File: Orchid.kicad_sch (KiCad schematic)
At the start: 122 parts, among them U1 nice_nano, U2 nice_nano

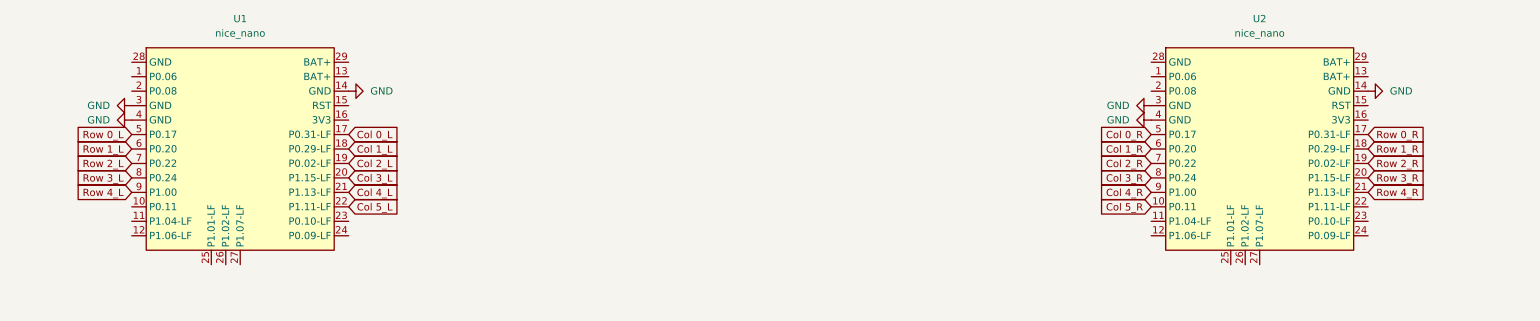
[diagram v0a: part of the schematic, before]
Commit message: Completed the diagram.
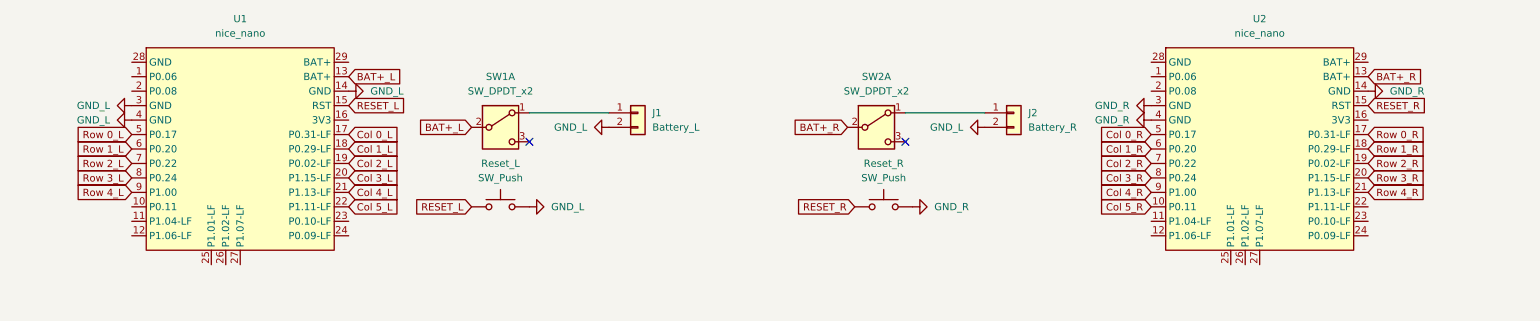
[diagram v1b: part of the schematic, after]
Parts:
- added J1: Battery_L, symbol Connector_Generic:Conn_01x02
- added J2: Battery_R, symbol Connector_Generic:Conn_01x02
- added Reset_L, Reset_R: SW_Push, symbol Switch:SW_Push
- added SW1, SW2: SW_DPDT_x2, symbol Switch:SW_DPDT_x2
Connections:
- net BAT+_R: now reaches U2.13 (BAT+)
- net BAT+_R: now also SW2.2 (B)
- net RESET_R: now reaches U2.15 (RST)
- net RESET_R: now also Reset_R.1
- net BAT+_L: now reaches U1.13 (BAT+)
- net BAT+_L: now also SW1.2 (B)
- net RESET_L: now reaches U1.15 (RST)
- net RESET_L: now also Reset_L.1
- net GND renamed GND_L
- net GND_L: now also J1.2 (Pin_2), J2.2 (Pin_2), Reset_L.2; no longer U2.14 (GND), U2.3 (GND), U2.4 (GND)
- new net: J2.1 (Pin_1), SW2.1 (A)
- new net: J1.1 (Pin_1), SW1.1 (A)
- new net GND_R: Reset_R.2, U2.14 (GND), U2.3 (GND), U2.4 (GND)
- no-connect marks 0 -> 2
